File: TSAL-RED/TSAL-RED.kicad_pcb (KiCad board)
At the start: 2 copper layers, 81.9 x 61.6 mm, 42 parts, among them J1 Conn_01x02, J2 Conn_01x02, J5 Conn_02x01, J6 Conn_02x03_Counter_Clockwise, K1 G5V-2, Q1 2N7002, Q2 AO3401A, U1 LM358, U2 4N35, U3 NE555D

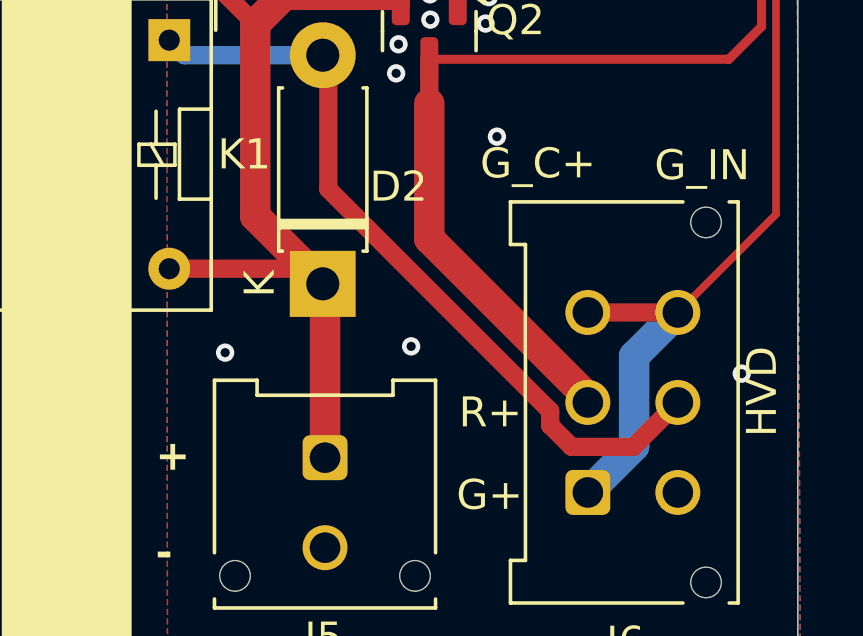
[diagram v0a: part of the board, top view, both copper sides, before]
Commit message: update check
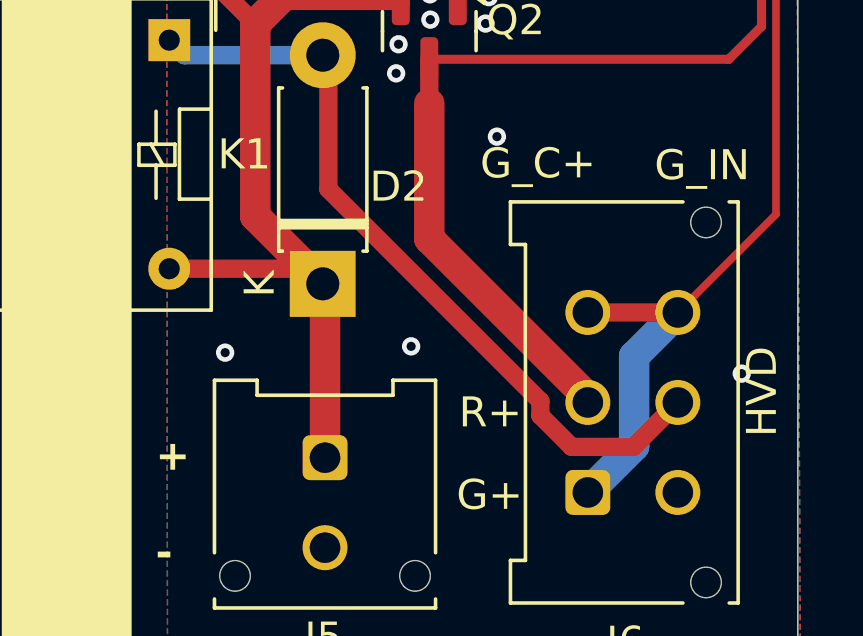
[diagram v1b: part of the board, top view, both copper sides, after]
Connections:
- J6 pad 4: unconnected-(J6-Pin_4-Pad4) -> GLV-
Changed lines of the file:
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@@
 	(net 30 "Net-(R4-Pad1)")
 	(net 31 "HVD_SDC_IN")
-	(net 32 "unconnected-(J6-Pin_4-Pad4)")
 	(footprint "Diode_THT:D_DO-41_SOD81_P7.62mm_Horizontal"
 		(layer "F.Cu")
@@
 			(layers "*.Cu" "*.Mask")
 			(remove_unused_layers no)
-			(net 32 "unconnected-(J6-Pin_4-Pad4)")
+			(net 1 "GLV-")
 			(pinfunction "Pin_4")
-			(pintype "passive+no_connect")
+			(pintype "passive")
 		)
 		(pad "5" thru_hole circle
@@
 	)
 	(segment
-		(start 125.570786 107.044214)
-		(end 127.630786 107.044214)
+		(start 124.528786 105.522214)
+		(end 124.528786 106.002214)
 		(width 0.6096)
 		(layer "F.Cu")
@@
 	(segment
 		(start 117.460786 98.454214)
-		(end 124.855986 105.849414)
+		(end 124.528786 105.522214)
 		(width 0.6096)
 		(layer "F.Cu")
@@
 	)
 	(segment
-		(start 117.460786 94.175786)
-		(end 117.460786 98.454214)
+		(start 124.528786 106.002214)
+		(end 125.570786 107.044214)
 		(width 0.6096)
 		(layer "F.Cu")
@@
 	)
 	(segment
-		(start 117.275 93.99)
-		(end 117.460786 94.175786)
+		(start 117.460786 94.175786)
+		(end 117.460786 98.454214)
 		(width 0.6096)
 		(layer "F.Cu")
@@
 	)
 	(segment
-		(start 124.855986 105.849414)
-		(end 124.855986 106.329414)
+		(start 125.570786 107.044214)
+		(end 127.630786 107.044214)
 		(width 0.6096)
 		(layer "F.Cu")
@@
 	)
 	(segment
-		(start 124.855986 106.329414)
-		(end 125.570786 107.044214)
+		(start 117.275 93.99)
+		(end 117.460786 94.175786)
 		(width 0.6096)
 		(layer "F.Cu")
